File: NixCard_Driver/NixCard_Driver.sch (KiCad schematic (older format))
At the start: 8 parts, among them P1 CONN_01X06, P2 CONN_01X06, P3 TSW-104-07-F-S, P4 TSW-104-07-F-S, U1 HV513WG, U2 HV513WG

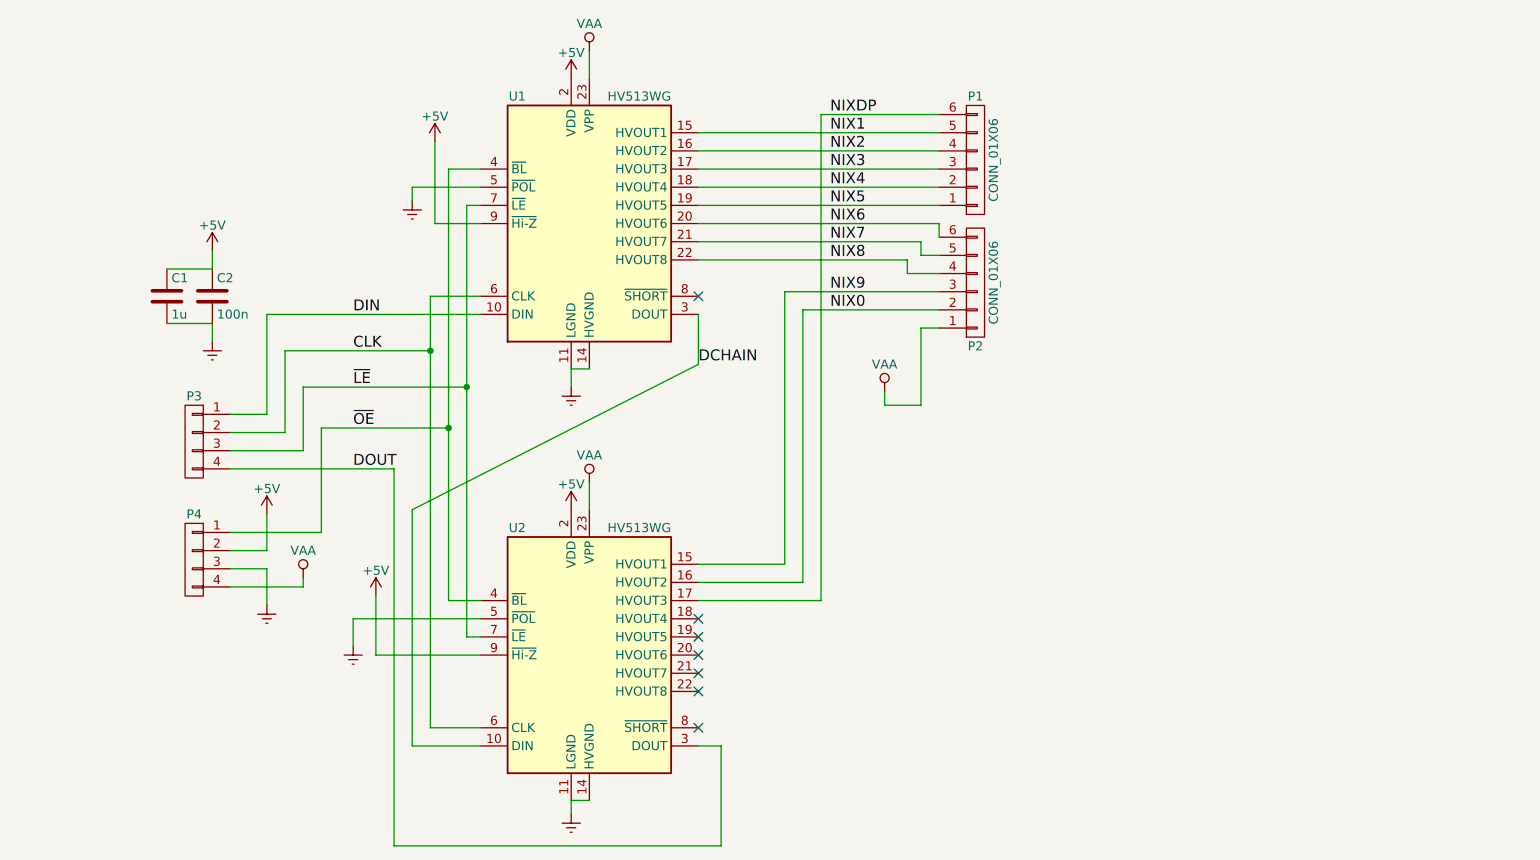
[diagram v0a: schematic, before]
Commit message: Redo of driver board
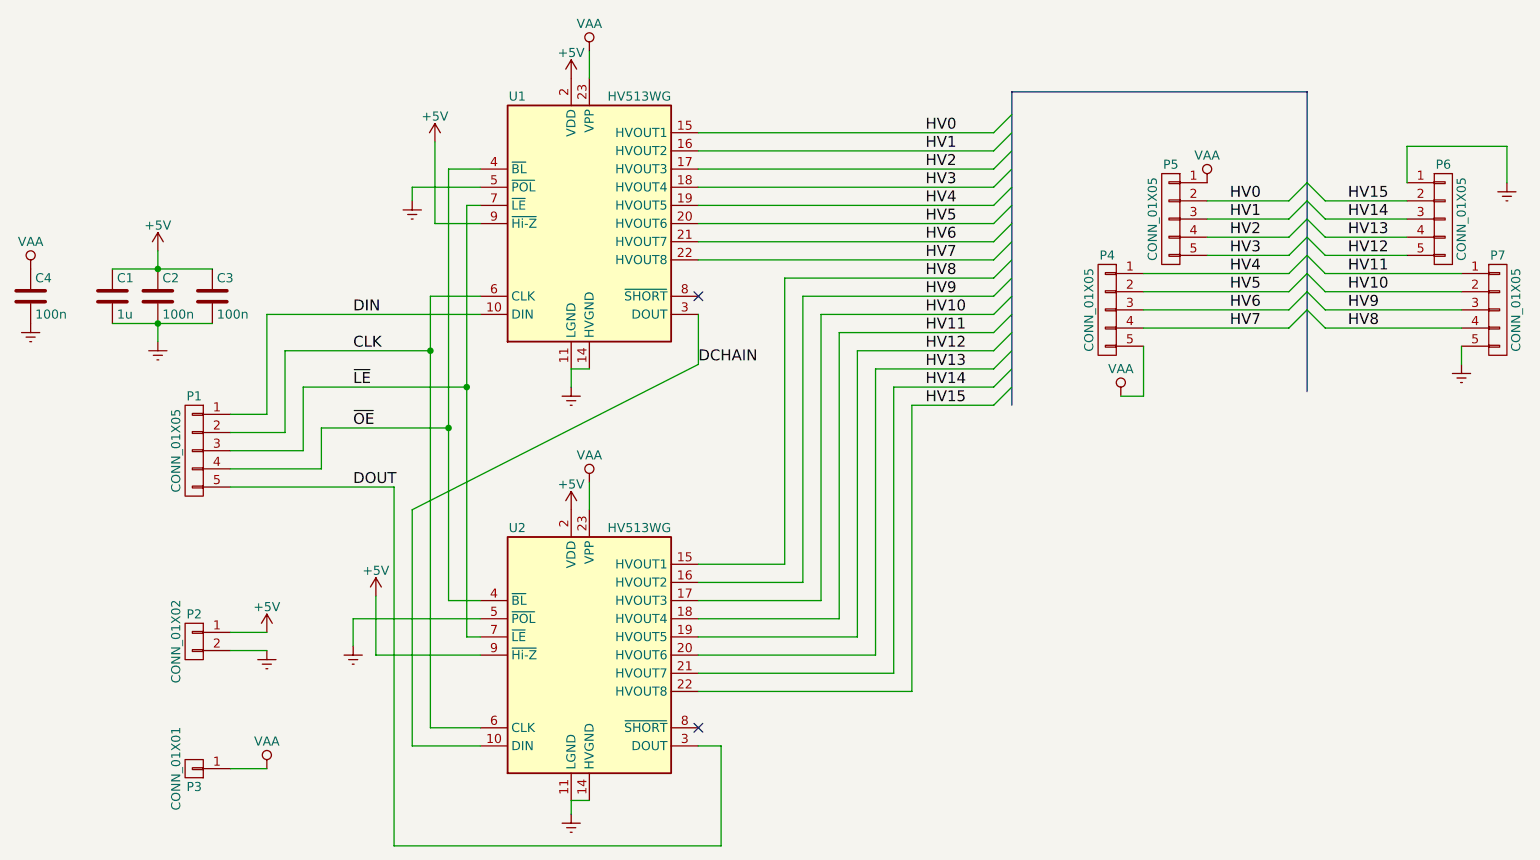
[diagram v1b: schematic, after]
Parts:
- removed P1, P2: CONN_01X06, Pin_Headers:Pin_Header_Straight_1x06_Pitch2.54mm, symbol CONN_01X06
- removed P3, P4: TSW-104-07-F-S, Pin_Headers:Pin_Header_Straight_1x04_Pitch2.54mm, symbol TSW-104-07-F-S
- added C3: 100n, Capacitors_SMD:C_0603, symbol 100n
- added C4: 100n, Capacitors_SMD:C_0805, symbol 100n
- added P1, P4, P5, P6, P7: CONN_01X05, Conn_PinHeader_2.54mm:PinHeader_1x05_P2.54mm_Vertical, symbol CONN_01X05
- added P2: CONN_01X02, Conn_PinHeader_2.54mm:PinHeader_1x02_P2.54mm_Vertical, symbol CONN_01X02
- added P3: CONN_01X01, Conn_PinHeader_2.54mm:PinHeader_1x01_P2.54mm_Vertical, symbol CONN_01X01
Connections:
- net +5V: now also C3.1, P2.1 (P1)
- net CLK: now also P1.2 (P2)
- net DIN: now also P1.1 (P1)
- net DOUT: now also P1.5 (P5)
- net GNDREF: now also C3.2, C4.2, P2.2 (P2), P6.1 (P1), P7.5 (P5)
- net VAA: now also C4.1, P3.1 (P1), P4.5 (P5), P5.1 (P1)
- net ~LE: now also P1.3 (P3)
- net ~OE: now also P1.4 (P4)
- net HV11: now reaches U2.18 (HVOUT4)
- net HV11: now also P7.1 (P1)
- net HV12: now reaches U2.19 (HVOUT5)
- net HV12: now also P6.5 (P5)
- net HV13: now reaches U2.20 (HVOUT6)
- net HV13: now also P6.4 (P4)
- net HV14: now reaches U2.21 (HVOUT7)
- net HV14: now also P6.3 (P3)
- net HV15: now reaches U2.22 (HVOUT8)
- net HV15: now also P6.2 (P2)
- net NIX0 renamed HV9
- net HV9: now also P7.3 (P3)
- net NIX1 renamed HV0
- net HV0: now also P5.2 (P2)
- net NIX2 renamed HV1
- net HV1: now also P5.3 (P3)
- net NIX3 renamed HV2
- net HV2: now also P5.4 (P4)
- net NIX4 renamed HV3
- net HV3: now also P5.5 (P5)
- net NIX5 renamed HV4
- net HV4: now also P4.1 (P1)
- net NIX6 renamed HV5
- net HV5: now also P4.2 (P2)
- net NIX7 renamed HV6
- net HV6: now also P4.3 (P3)
- net NIX8 renamed HV7
- net HV7: now also P4.4 (P4)
- net NIX9 renamed HV8
- net HV8: now also P7.4 (P4)
- net NIXDP renamed HV10
- net HV10: now also P7.2 (P2)
- no-connect marks 7 -> 2
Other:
- moved on the sheet: C1, C2
